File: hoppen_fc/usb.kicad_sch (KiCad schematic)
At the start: 10 parts, among them J2 USB_C_Receptacle_USB2.0_16P, U10 USBLC6-2SC6

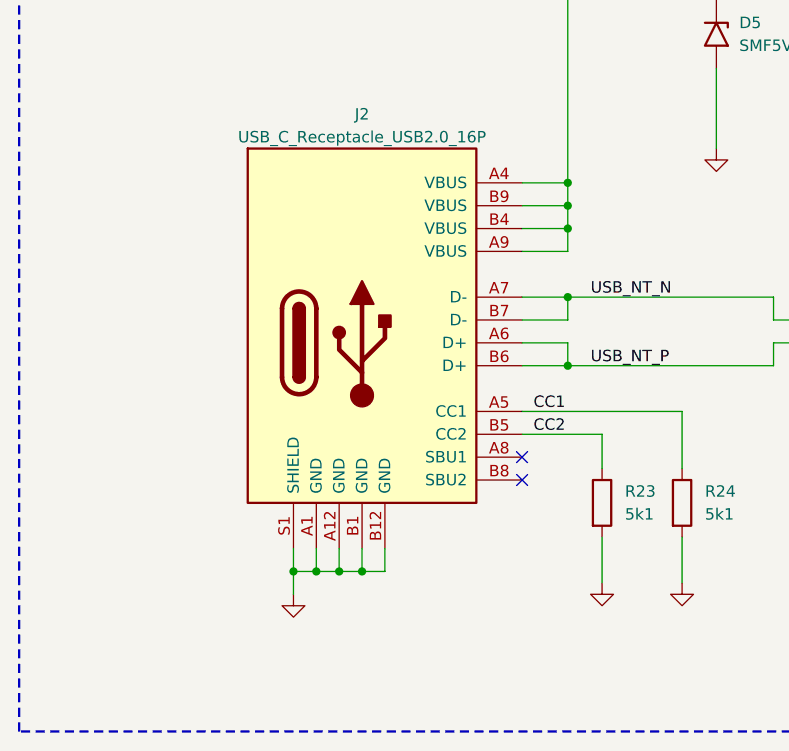
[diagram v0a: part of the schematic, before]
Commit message: ready for routing?
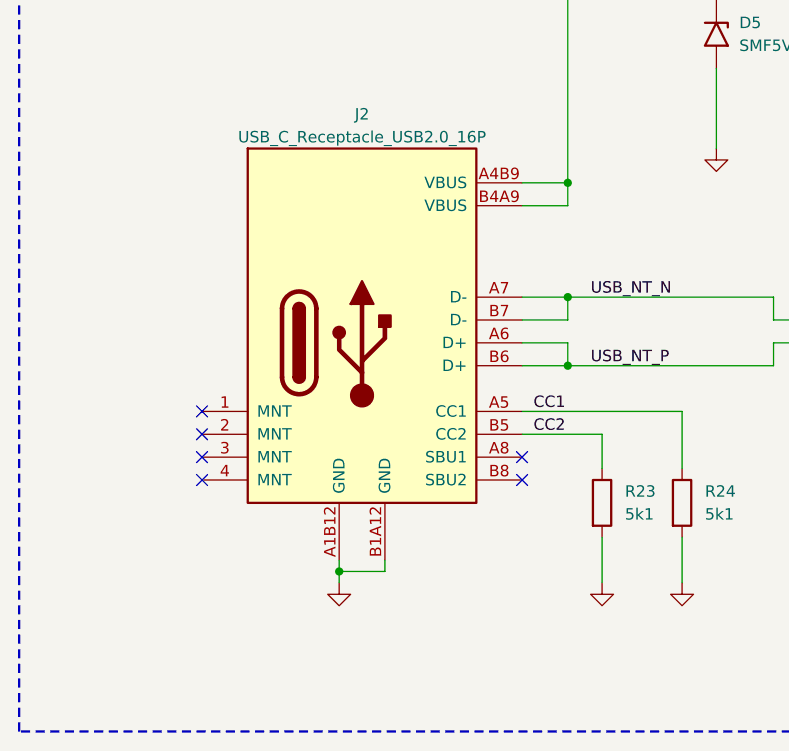
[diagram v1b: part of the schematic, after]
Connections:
- net +VBUS: now also J2.A4B9 (VBUS), J2.B4A9 (VBUS); no longer J2.A4 (VBUS), J2.A9 (VBUS), J2.B4 (VBUS), J2.B9 (VBUS)
- net GND: now also J2.A1B12 (GND), J2.B1A12 (GND); no longer J2.A1 (GND), J2.A12 (GND), J2.B1 (GND), J2.B12 (GND), J2.S1 (SHIELD)
- no-connect marks 2 -> 6
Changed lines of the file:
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@@
-	)
-	(junction
-		(at 109.22 134.62)
-		(diameter 0)
-		(color 0 0 0 0)
 	)
 	(junction
@@
 	)
 	(junction
-		(at 114.3 134.62)
-		(diameter 0)
-		(color 0 0 0 0)
-	)
-	(junction
-		(at 106.68 134.62)
-		(diameter 0)
-		(color 0 0 0 0)
-	)
-	(junction
 		(at 171.45 86.36)
 		(diameter 0)
@@
 	)
 	(junction
-		(at 137.16 63.5)
+		(at 111.76 134.62)
 		(diameter 0)
 		(color 0 0 0 0)
 	)
 	(junction
-		(at 137.16 96.52)
-		(diameter 0)
-		(color 0 0 0 0)
-	)
-	(junction
-		(at 111.76 134.62)
+		(at 137.16 63.5)
 		(diameter 0)
 		(color 0 0 0 0)
@@
 	)
 	(junction
-		(at 137.16 93.98)
-		(diameter 0)
-		(color 0 0 0 0)
-	)
-	(junction
 		(at 153.67 63.5)
 		(diameter 0)
@@
 	)
 	(no_connect
+		(at 96.52 124.46)
+	)
+	(no_connect
+		(at 96.52 121.92)
+	)
+	(no_connect
 		(at 132.08 121.92)
+	)
+	(no_connect
+		(at 96.52 116.84)
+	)
+	(no_connect
+		(at 96.52 119.38)
 	)
 	(no_connect
@@
 	(wire
 		(pts
+			(xy 111.76 133.35) (xy 111.76 134.62)
+		)
+		(stroke
+			(width 0)
+			(type default)
+		)
+	)
+	(wire
+		(pts
 			(xy 167.64 114.3) (xy 167.64 118.11)
 		)
@@
 	(wire
 		(pts
-			(xy 116.84 132.08) (xy 116.84 134.62)
-		)
-		(stroke
-			(width 0)
-			(type default)
-		)
-	)
-	(wire
-		(pts
-			(xy 106.68 132.08) (xy 106.68 134.62)
-		)
-		(stroke
-			(width 0)
-			(type default)
-		)
-	)
-	(wire
-		(pts
 			(xy 181.61 74.93) (xy 187.96 74.93)
 		)
@@
 	(wire
 		(pts
-			(xy 106.68 134.62) (xy 109.22 134.62)
-		)
-		(stroke
-			(width 0)
-			(type default)
-		)
-	)
-	(wire
-		(pts
 			(xy 160.02 109.22) (xy 162.56 109.22)
 		)
@@
 	(wire
 		(pts
-			(xy 106.68 134.62) (xy 106.68 137.16)
-		)
-		(stroke
-			(width 0)
-			(type default)
-		)
-	)
-	(wire
-		(pts
-			(xy 111.76 134.62) (xy 114.3 134.62)
-		)
-		(stroke
-			(width 0)
-			(type default)
-		)
-	)
-	(wire
-		(pts
 			(xy 137.16 104.14) (xy 132.08 104.14)
 		)
@@
 	(wire
 		(pts
-			(xy 116.84 134.62) (xy 114.3 134.62)
-		)
-		(stroke
-			(width 0)
-			(type default)
-		)
-	)
-	(wire
-		(pts
 			(xy 153.67 63.5) (xy 171.45 63.5)
 		)
@@
 	(wire
 		(pts
-			(xy 137.16 96.52) (xy 137.16 93.98)
-		)
-		(stroke
-			(width 0)
-			(type default)
-		)
-	)
-	(wire
-		(pts
 			(xy 132.08 111.76) (xy 137.16 111.76)
 		)
@@
 	(wire
 		(pts
-			(xy 111.76 132.08) (xy 111.76 134.62)
-		)
-		(stroke
-			(width 0)
-			(type default)
-		)
-	)
-	(wire
-		(pts
 			(xy 137.16 63.5) (xy 137.16 91.44)
 		)
@@
 	(wire
 		(pts
-			(xy 132.08 96.52) (xy 137.16 96.52)
-		)
-		(stroke
-			(width 0)
-			(type default)
-		)
-	)
-	(wire
-		(pts
-			(xy 109.22 134.62) (xy 111.76 134.62)
-		)
-		(stroke
-			(width 0)
-			(type default)
-		)
-	)
-	(wire
-		(pts
 			(xy 160.02 106.68) (xy 162.56 106.68)
 		)
@@
 	(wire
 		(pts
-			(xy 109.22 132.08) (xy 109.22 134.62)
-		)
-		(stroke
-			(width 0)
-			(type default)
-		)
-	)
-	(wire
-		(pts
-			(xy 132.08 99.06) (xy 137.16 99.06)
-		)
-		(stroke
-			(width 0)
-			(type default)
-		)
-	)
-	(wire
-		(pts
-			(xy 114.3 132.08) (xy 114.3 134.62)
+			(xy 116.84 134.62) (xy 111.76 134.62)
 		)
 		(stroke
@@
 	(wire
 		(pts
+			(xy 116.84 133.35) (xy 116.84 134.62)
+		)
+		(stroke
+			(width 0)
+			(type default)
+		)
+	)
+	(wire
+		(pts
 			(xy 137.16 58.42) (xy 137.16 63.5)
 		)
@@
 	(wire
 		(pts
-			(xy 137.16 99.06) (xy 137.16 96.52)
-		)
-		(stroke
-			(width 0)
-			(type default)
-		)
-	)
-	(wire
-		(pts
 			(xy 160.02 104.14) (xy 160.02 106.68)
 		)
@@
 		(pts
 			(xy 137.16 111.76) (xy 137.16 109.22)
+		)
+		(stroke
+			(width 0)
+			(type default)
+		)
+	)
+	(wire
+		(pts
+			(xy 111.76 134.62) (xy 111.76 135.89)
 		)
 		(stroke
@@
 	)
 	(symbol
+		(lib_id "power:GND")
+		(at 111.76 135.89 0)
+		(unit 1)
+		(exclude_from_sim no)
+		(in_bom yes)
+		(on_board yes)
+		(dnp no)
+		(fields_autoplaced yes)
+		(property "Reference" "#PWR089"
+			(at 111.76 142.24 0)
+			(effects
+				(font
+					(size 1.27 1.27)
+				)
+				(hide yes)
+			)
+		)
+		(property "Value" "GND"
+			(at 111.76 140.97 0)
+			(effects
+				(font
+					(size 1.27 1.27)
+				)
+				(hide yes)
+			)
+		)
+		(property "Footprint" ""
+			(at 111.76 135.89 0)
+			(effects
+				(font
+					(size 1.27 1.27)
+				)
+				(hide yes)
+			)
+		)
+		(property "Datasheet" ""
+			(at 111.76 135.89 0)
+			(effects
+				(font
+					(size 1.27 1.27)
+				)
+				(hide yes)
+			)
+		)
+		(property "Description" "Power symbol creates a global label with name \"GND\" , ground"
+			(at 111.76 135.89 0)
+			(effects
+				(font
+					(size 1.27 1.27)
+				)
+				(hide yes)
+			)
+		)
+		(pin "1"
+		)
+		(instances
+			(project "hoppen_fc"
+				(path "/abe950a1-9eef-4508-9fd4-31d3e723e029/c85454e5-a89e-41eb-a5ed-71b4fc4cf13a/70185383-c6d2-4eb6-9764-fd02002b35f8"
+					(reference "#PWR089")
+					(unit 1)
+				)
+			)
+		)
+	)
+	(symbol
 		(lib_id "0_connectors:USB_C_Receptacle_USB2.0_16P")
 		(at 114.3 109.22 0)
@@
 			)
 		)
-		(pin "B1"
+		(pin "A4B9"
 		)
 		(pin "A5"
@@
 		(pin "A7"
 		)
-		(pin "A12"
-		)
-		(pin "A4"
-		)
-		(pin "A9"
-		)
-		(pin "B12"
-		)
-		(pin "S1"
-		)
-		(pin "B9"
-		)
-		(pin "A1"
-		)
-		(pin "B4"
+		(pin "B1A12"
+		)
+		(pin "2"
+		)
+		(pin "3"
+		)
+		(pin "4"
+		)
+		(pin "B4A9"
+		)
+		(pin "1"
+		)
+		(pin "A1B12"
 		)
 		(pin "B5"
@@
 					(unit 1)
 				)
-			)
-		)
-	)
-	(symbol
-		(lib_id "power:GND")
-		(at 106.68 137.16 0)
-		(unit 1)
-		(exclude_from_sim no)
-		(in_bom yes)
-		(on_board yes)
-		(dnp no)
-		(fields_autoplaced yes)
-		(property "Reference" "#PWR089"
-			(at 106.68 143.51 0)
-			(effects
-				(font
-					(size 1.27 1.27)
-				)
-				(hide yes)
-			)
-		)
-		(property "Value" "GND"
-			(at 106.68 142.24 0)
-			(effects
-				(font
-					(size 1.27 1.27)
-				)
-				(hide yes)
-			)
-		)
-		(property "Footprint" ""
-			(at 106.68 137.16 0)
-			(effects
-				(font
-					(size 1.27 1.27)
-				)
-				(hide yes)
-			)
-		)
-		(property "Datasheet" ""
-			(at 106.68 137.16 0)
-			(effects
-				(font
-					(size 1.27 1.27)
-				)
-				(hide yes)
-			)
-		)
-		(property "Description" "Power symbol creates a global label with name \"GND\" , ground"
-			(at 106.68 137.16 0)
-			(effects
-				(font
-					(size 1.27 1.27)
-				)
-				(hide yes)
-			)
-		)
-		(pin "1"
-		)
-		(instances
-			(project "hoppen_fc"
-				(path "/abe950a1-9eef-4508-9fd4-31d3e723e029/c85454e5-a89e-41eb-a5ed-71b4fc4cf13a/70185383-c6d2-4eb6-9764-fd02002b35f8"
-					(reference "#PWR089")
-					(unit 1)
-				)
